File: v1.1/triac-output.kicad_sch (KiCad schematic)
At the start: 7 parts, among them Q3 T835-600B, Q4 2N7002, U6 TLP160G

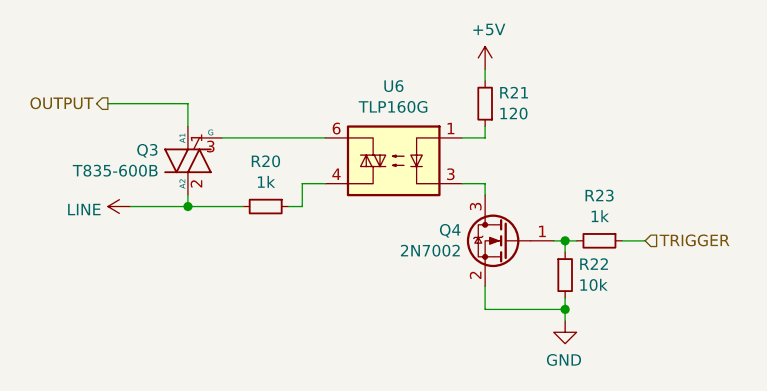
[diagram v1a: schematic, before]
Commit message: more routing
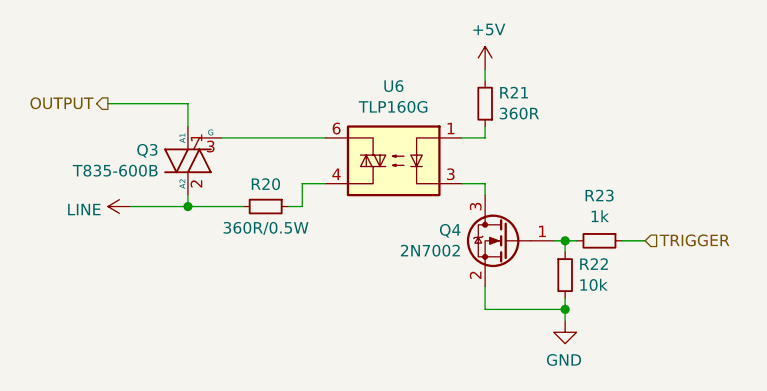
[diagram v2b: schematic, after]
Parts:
- R20: value 1k -> 360R/0.5W; Part (none) -> Panasonic ERJP08F3600V
- R21: value 120 -> 360R
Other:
- title: (none) -> MadPresso controller
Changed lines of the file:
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@@
   (page 0 6)
   (paper "A5")
+  (title_block
+    (title "MadPresso controller")
+    (date "2020-11-18")
+    (rev "1.1")
+  )
   (junction (at 91.44 57.15) (diameter 1.016) (color 0 0 0 0))
   (junction (at 133.35 60.96) (diameter 1.016) (color 0 0 0 0))
@@
   (symbol (lib_id "power:LINE") (at 85.09 57.15 90) (mirror x)
     (in_bom yes) (on_board yes)
-    (property "Reference" "#PWR051" (id 0) (at 88.9 57.15 0)
+    (property "Reference" "#PWR045" (id 0) (at 88.9 57.15 0)
       (effects (font (size 1.27 1.27)) hide)
     )
@@
   (symbol (lib_id "power:+5V") (at 124.46 41.91 0)
     (in_bom yes) (on_board yes)
-    (property "Reference" "#PWR052" (id 0) (at 124.46 45.72 0)
+    (property "Reference" "#PWR046" (id 0) (at 124.46 45.72 0)
       (effects (font (size 1.27 1.27)) hide)
     )
@@
   (symbol (lib_id "power:GND") (at 133.35 69.85 0) (mirror y)
     (in_bom yes) (on_board yes)
-    (property "Reference" "#PWR053" (id 0) (at 133.35 76.2 0)
+    (property "Reference" "#PWR047" (id 0) (at 133.35 76.2 0)
       (effects (font (size 1.27 1.27)) hide)
     )
@@
   (symbol (lib_id "Device:R_Small") (at 100.076 57.15 270)
     (in_bom yes) (on_board yes)
-    (property "Reference" "R20" (id 0) (at 100.076 52.1716 90))
-    (property "Value" "1k" (id 1) (at 100.076 54.483 90))
+    (property "Reference" "R20" (id 0) (at 100.076 54.7116 90))
+    (property "Value" "360R/0.5W" (id 1) (at 100.076 59.563 90))
     (property "Footprint" "Resistor_SMD:R_1206_3216Metric_Pad1.30x1.75mm_HandSolder" (id 2) (at 100.076 57.15 0)
       (effects (font (size 1.27 1.27)) hide)
     )
-    (property "Datasheet" "~" (id 3) (at 100.076 57.15 0)
+    (property "Datasheet" "https://docs.rs-online.com/ef78/0900766b812cb812.pdf" (id 3) (at 100.076 57.15 0)
+      (effects (font (size 1.27 1.27)) hide)
+    )
+    (property "Part" "Panasonic ERJP08F3600V" (id 4) (at 100.076 57.15 90)
       (effects (font (size 1.27 1.27)) hide)
     )
@@
       (effects (font (size 1.27 1.27)) (justify right))
     )
-    (property "Value" "120" (id 1) (at 125.9586 46.863 0)
+    (property "Value" "360R" (id 1) (at 125.9586 46.863 0)
       (effects (font (size 1.27 1.27)) (justify right))
     )
